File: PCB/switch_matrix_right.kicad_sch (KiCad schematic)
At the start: 78 parts, among them SW41 SW_Push, SW42 SW_Push, SW43 SW_Push, SW44 SW_Push, SW45 SW_Push, SW46 SW_Push, SW47 SW_Push, SW48 SW_Push, SW49 SW_Push, SW50 SW_Push, SW51 SW_Push, SW52 SW_Push, SW53 SW_Push, SW54 SW_Push, SW55 SW_Push, SW56 SW_Push, SW57 SW_Push, SW58 SW_Push, SW59 SW_Push, SW60 SW_Push, SW61 SW_Push, SW62 SW_Push, SW63 SW_Push, SW64 SW_Push, SW65 SW_Push, SW66 SW_Push, SW67 SW_Push, SW68 SW_Push, SW69 SW_Push, SW70 SW_Push, SW71 SW_Push, SW72 SW_Push, SW73 SW_Push, SW74 SW_Push, SW75 SW_Push, SW76 SW_Push, SW77 SW_Push, SW78 SW_Push, SW79 SW_Push

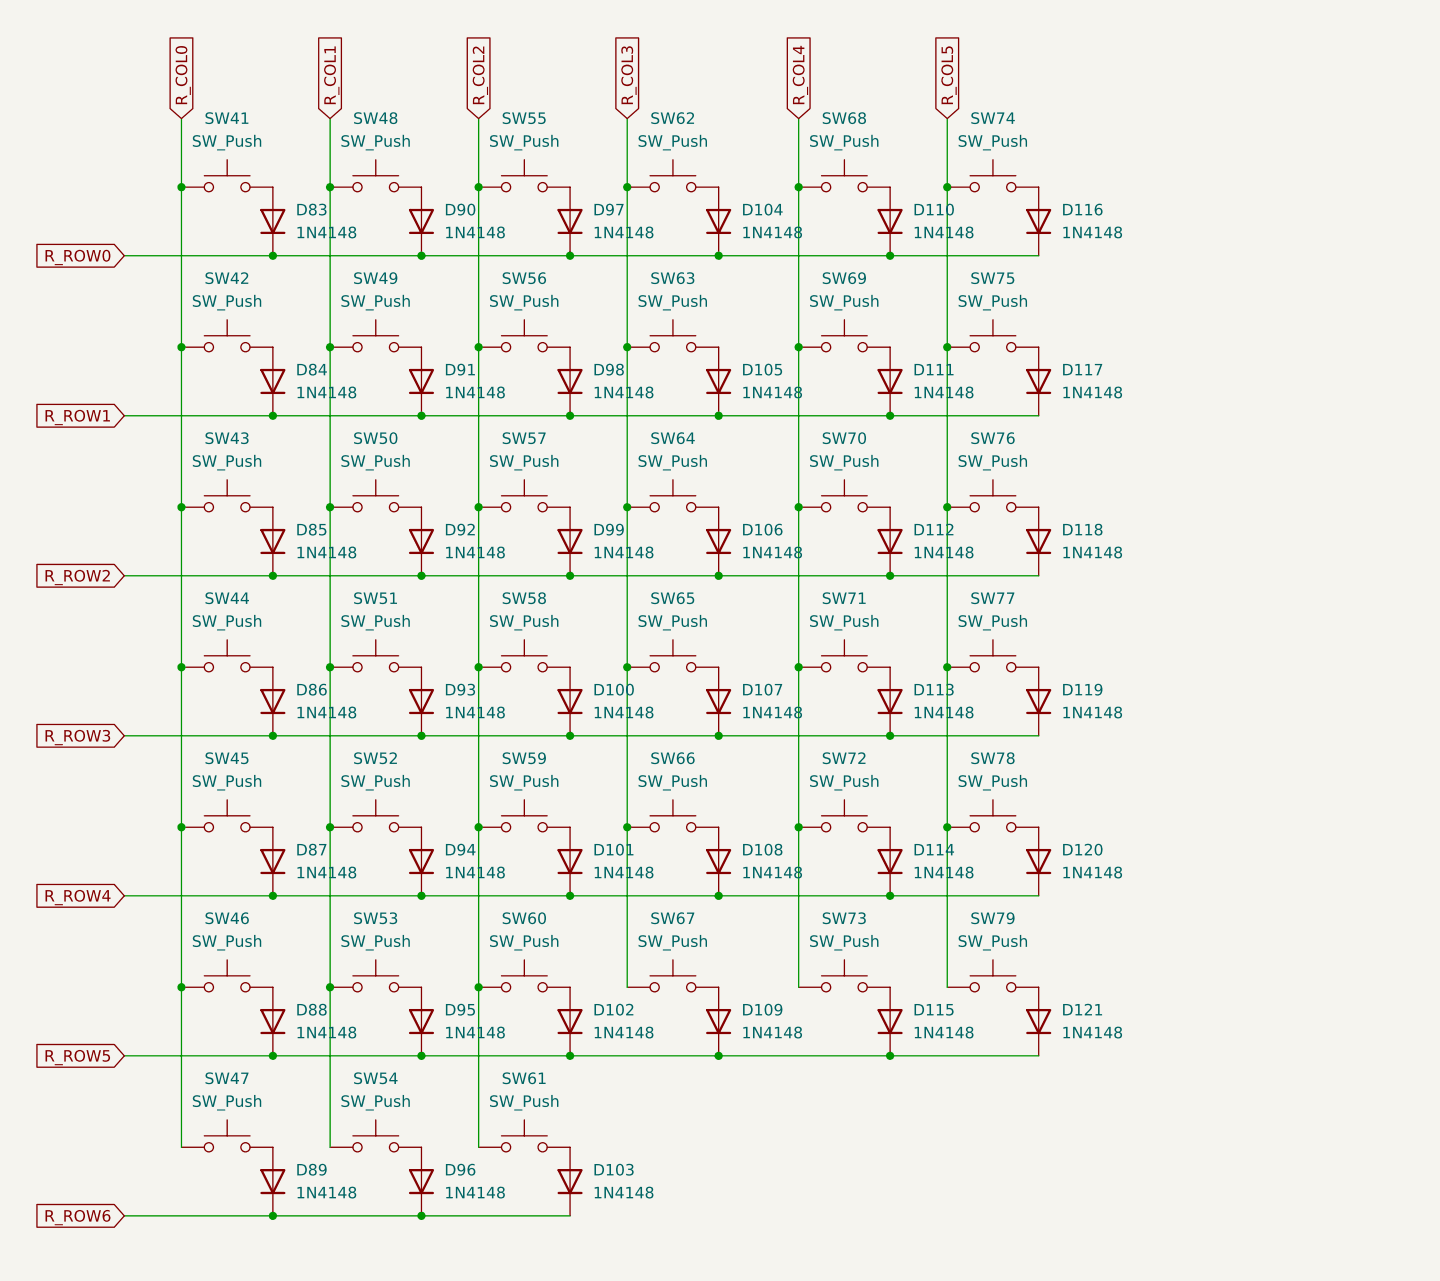
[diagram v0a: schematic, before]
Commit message: updated schematic
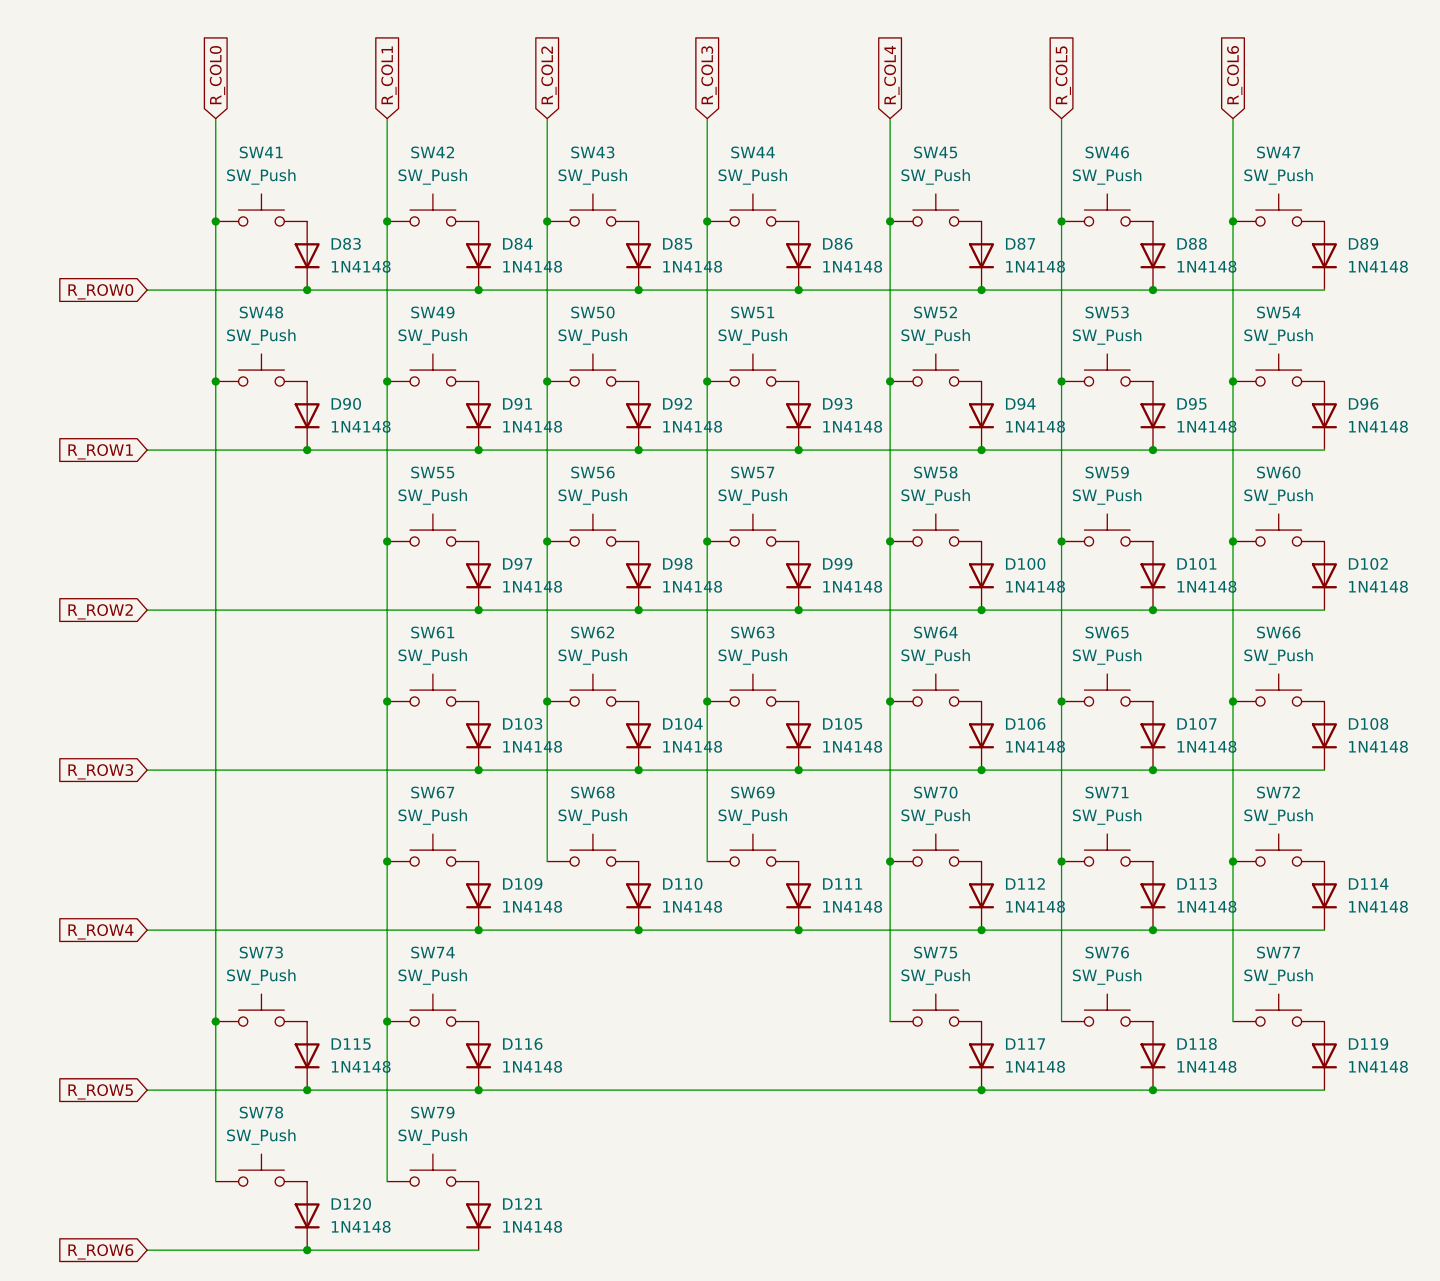
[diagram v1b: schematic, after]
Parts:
- SW41, SW42, SW43, SW44, SW45, SW46, SW47, SW48, SW49, SW50, SW51, SW52, SW53, SW54, SW55, SW56, SW57, SW58, SW59, SW62, SW63, SW64, SW65, SW66, SW67, SW68, SW69, SW70, SW71, SW72, SW73, SW74, SW75: footprint Gateron_KS33_Hotswap:Gateron-KS33-Hotswap-1U -> (none)
- SW60, SW61: footprint Gateron_KS33_Hotswap:Gateron-KS33-Hotswap-2U -> (none)
- SW76, SW77, SW78, SW79: footprint Gateron_KS33_Hotswap:Gateron-KS33-Hotswap-1.25U -> (none)
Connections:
- net R_COL0: now also SW48.1, SW73.1, SW78.1; no longer SW42.1, SW43.1, SW44.1, SW45.1, SW46.1, SW47.1
- net R_COL1: now also SW42.1, SW55.1, SW61.1, SW67.1, SW74.1, SW79.1; no longer SW48.1, SW50.1, SW51.1, SW52.1, SW53.1, SW54.1
- net R_COL2: now also SW43.1, SW50.1, SW62.1, SW68.1; no longer SW55.1, SW57.1, SW58.1, SW59.1, SW60.1, SW61.1
- net R_COL3: now also SW44.1, SW51.1, SW57.1, SW69.1; no longer SW62.1, SW64.1, SW65.1, SW66.1, SW67.1
- net R_COL4: now also SW45.1, SW52.1, SW58.1, SW64.1, SW75.1; no longer SW68.1, SW69.1, SW71.1, SW72.1, SW73.1
- net R_COL5: now also SW46.1, SW53.1, SW59.1, SW65.1, SW71.1; no longer SW74.1, SW75.1, SW77.1, SW78.1, SW79.1
- net R_ROW0: now also D84.1 (K), D85.1 (K), D86.1 (K), D87.1 (K), D88.1 (K), D89.1 (K); no longer D104.1 (K), D110.1 (K), D116.1 (K), D90.1 (K), D97.1 (K)
- net R_ROW1: now also D90.1 (K), D92.1 (K), D93.1 (K), D94.1 (K), D95.1 (K), D96.1 (K); no longer D105.1 (K), D111.1 (K), D117.1 (K), D84.1 (K), D98.1 (K)
- net R_ROW2: now also D100.1 (K), D101.1 (K), D102.1 (K), D97.1 (K), D98.1 (K); no longer D106.1 (K), D112.1 (K), D118.1 (K), D85.1 (K), D92.1 (K)
- net R_ROW3: now also D103.1 (K), D104.1 (K), D105.1 (K), D106.1 (K), D108.1 (K); no longer D100.1 (K), D113.1 (K), D119.1 (K), D86.1 (K), D93.1 (K)
- net R_ROW4: now also D109.1 (K), D110.1 (K), D111.1 (K), D112.1 (K), D113.1 (K); no longer D101.1 (K), D108.1 (K), D120.1 (K), D87.1 (K), D94.1 (K)
- net R_ROW5: now also D116.1 (K), D117.1 (K), D118.1 (K), D119.1 (K); no longer D102.1 (K), D109.1 (K), D121.1 (K), D88.1 (K), D95.1 (K)
- net R_ROW6: now also D120.1 (K), D121.1 (K); no longer D103.1 (K), D89.1 (K), D96.1 (K)
- new net R_COL6: SW47.1, SW54.1, SW60.1, SW66.1, SW72.1, SW77.1

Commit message: routed the switches and diodes
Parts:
- SW41, SW42, SW43, SW44, SW45, SW46, SW47, SW48, SW49, SW50, SW51, SW52, SW53, SW54, SW55, SW56, SW57, SW58, SW59, SW61, SW62, SW63, SW64, SW65, SW67, SW68, SW69, SW70, SW71, SW74, SW75, SW76, SW79: footprint (none) -> Gateron_KS33_Hotswap:Gateron-KS33-Hotswap-1U
- SW60, SW66, SW72, SW77: footprint (none) -> Gateron_KS33_Hotswap:Gateron-KS33-Hotswap-1.25U
- SW73, SW78: footprint (none) -> Gateron_KS33_Hotswap:Gateron-KS33-Hotswap-2U
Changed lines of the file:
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@@
 			)
 		)
-		(property "Footprint" ""
+		(property "Footprint" "Gateron_KS33_Hotswap:Gateron-KS33-Hotswap-1U"
 			(at 96.52 30.48 0)
 			(effects
@@
 			)
 		)
-		(property "Footprint" ""
+		(property "Footprint" "Gateron_KS33_Hotswap:Gateron-KS33-Hotswap-1U"
 			(at 116.84 30.48 0)
 			(effects
@@
 			)
 		)
-		(property "Footprint" ""
+		(property "Footprint" "Gateron_KS33_Hotswap:Gateron-KS33-Hotswap-1U"
 			(at 135.89 66.04 0)
 			(effects
@@
 			)
 		)
-		(property "Footprint" ""
+		(property "Footprint" "Gateron_KS33_Hotswap:Gateron-KS33-Hotswap-1U"
 			(at 96.52 66.04 0)
 			(effects
@@
 			)
 		)
-		(property "Footprint" ""
+		(property "Footprint" "Gateron_KS33_Hotswap:Gateron-KS33-Hotswap-1U"
 			(at 116.84 48.26 0)
 			(effects
@@
 			)
 		)
-		(property "Footprint" ""
+		(property "Footprint" "Gateron_KS33_Hotswap:Gateron-KS33-Hotswap-1U"
 			(at 96.52 83.82 0)
 			(effects
@@
 			)
 		)
-		(property "Footprint" ""
+		(property "Footprint" "Gateron_KS33_Hotswap:Gateron-KS33-Hotswap-1U"
 			(at 78.74 83.82 0)
 			(effects
@@
 			)
 		)
-		(property "Footprint" ""
+		(property "Footprint" "Gateron_KS33_Hotswap:Gateron-KS33-Hotswap-2U"
 			(at 41.91 137.16 0)
 			(effects
@@
 			)
 		)
-		(property "Footprint" ""
+		(property "Footprint" "Gateron_KS33_Hotswap:Gateron-KS33-Hotswap-1U"
 			(at 135.89 83.82 0)
 			(effects
@@
 			)
 		)
-		(property "Footprint" ""
+		(property "Footprint" "Gateron_KS33_Hotswap:Gateron-KS33-Hotswap-1U"
 			(at 116.84 66.04 0)
 			(effects
@@
 			)
 		)
-		(property "Footprint" ""
+		(property "Footprint" "Gateron_KS33_Hotswap:Gateron-KS33-Hotswap-1U"
 			(at 135.89 30.48 0)
 			(effects
@@
 			)
 		)
-		(property "Footprint" ""
+		(property "Footprint" "Gateron_KS33_Hotswap:Gateron-KS33-Hotswap-1.25U"
 			(at 154.94 119.38 0)
 			(effects
@@
 			)
 		)
-		(property "Footprint" ""
+		(property "Footprint" "Gateron_KS33_Hotswap:Gateron-KS33-Hotswap-1U"
 			(at 60.96 66.04 0)
 			(effects
@@
 			)
 		)
-		(property "Footprint" ""
+		(property "Footprint" "Gateron_KS33_Hotswap:Gateron-KS33-Hotswap-1U"
 			(at 96.52 48.26 0)
 			(effects
@@
 			)
 		)
-		(property "Footprint" ""
+		(property "Footprint" "Gateron_KS33_Hotswap:Gateron-KS33-Hotswap-1U"
 			(at 60.96 137.16 0)
 			(effects
@@
 			)
 		)
-		(property "Footprint" ""
+		(property "Footprint" "Gateron_KS33_Hotswap:Gateron-KS33-Hotswap-1U"
 			(at 116.84 119.38 0)
 			(effects
@@
 			)
 		)
-		(property "Footprint" ""
+		(property "Footprint" "Gateron_KS33_Hotswap:Gateron-KS33-Hotswap-1U"
 			(at 116.84 101.6 0)
 			(effects
@@
 			)
 		)
-		(property "Footprint" ""
+		(property "Footprint" "Gateron_KS33_Hotswap:Gateron-KS33-Hotswap-1U"
 			(at 60.96 119.38 0)
 			(effects
@@
 			)
 		)
-		(property "Footprint" ""
+		(property "Footprint" "Gateron_KS33_Hotswap:Gateron-KS33-Hotswap-1U"
 			(at 60.96 83.82 0)
 			(effects
@@
 			)
 		)
-		(property "Footprint" ""
+		(property "Footprint" "Gateron_KS33_Hotswap:Gateron-KS33-Hotswap-1U"
 			(at 78.74 30.48 0)
 			(effects
@@
 			)
 		)
-		(property "Footprint" ""
+		(property "Footprint" "Gateron_KS33_Hotswap:Gateron-KS33-Hotswap-1U"
 			(at 135.89 101.6 0)
 			(effects
@@
 			)
 		)
-		(property "Footprint" ""
+		(property "Footprint" "Gateron_KS33_Hotswap:Gateron-KS33-Hotswap-1.25U"
 			(at 154.94 101.6 0)
 			(effects
@@
 			)
 		)
-		(property "Footprint" ""
+		(property "Footprint" "Gateron_KS33_Hotswap:Gateron-KS33-Hotswap-1U"
 			(at 116.84 83.82 0)
 			(effects
@@
 			)
 		)
-		(property "Footprint" ""
+		(property "Footprint" "Gateron_KS33_Hotswap:Gateron-KS33-Hotswap-2U"
 			(at 41.91 119.38 0)
 			(effects
@@
 			)
 		)
-		(property "Footprint" ""
+		(property "Footprint" "Gateron_KS33_Hotswap:Gateron-KS33-Hotswap-1.25U"
 			(at 154.94 66.04 0)
 			(effects
@@
 			)
 		)
-		(property "Footprint" ""
+		(property "Footprint" "Gateron_KS33_Hotswap:Gateron-KS33-Hotswap-1U"
 			(at 78.74 101.6 0)
 			(effects
@@
 			)
 		)
-		(property "Footprint" ""
+		(property "Footprint" "Gateron_KS33_Hotswap:Gateron-KS33-Hotswap-1U"
 			(at 135.89 48.26 0)
 			(effects
@@
 			)
 		)
-		(property "Footprint" ""
+		(property "Footprint" "Gateron_KS33_Hotswap:Gateron-KS33-Hotswap-1.25U"
 			(at 154.94 83.82 0)
 			(effects
@@
 			)
 		)
-		(property "Footprint" ""
+		(property "Footprint" "Gateron_KS33_Hotswap:Gateron-KS33-Hotswap-1U"
 			(at 78.74 66.04 0)
 			(effects
@@
 			)
 		)
-		(property "Footprint" ""
+		(property "Footprint" "Gateron_KS33_Hotswap:Gateron-KS33-Hotswap-1U"
 			(at 96.52 101.6 0)
 			(effects
@@
 			)
 		)
-		(property "Footprint" ""
+		(property "Footprint" "Gateron_KS33_Hotswap:Gateron-KS33-Hotswap-1U"
 			(at 154.94 48.26 0)
 			(effects
@@
 			)
 		)
-		(property "Footprint" ""
+		(property "Footprint" "Gateron_KS33_Hotswap:Gateron-KS33-Hotswap-1U"
 			(at 154.94 30.48 0)
 			(effects
@@
 			)
 		)
-		(property "Footprint" ""
+		(property "Footprint" "Gateron_KS33_Hotswap:Gateron-KS33-Hotswap-1U"
 			(at 78.74 48.26 0)
 			(effects
@@
 			)
 		)
-		(property "Footprint" ""
+		(property "Footprint" "Gateron_KS33_Hotswap:Gateron-KS33-Hotswap-1U"
 			(at 60.96 48.26 0)
 			(effects
@@
 			)
 		)
-		(property "Footprint" ""
+		(property "Footprint" "Gateron_KS33_Hotswap:Gateron-KS33-Hotswap-1U"
 			(at 41.91 48.26 0)
 			(effects
@@
 			)
 		)
-		(property "Footprint" ""
+		(property "Footprint" "Gateron_KS33_Hotswap:Gateron-KS33-Hotswap-1U"
 			(at 135.89 119.38 0)
 			(effects
@@
 			)
 		)
-		(property "Footprint" ""
+		(property "Footprint" "Gateron_KS33_Hotswap:Gateron-KS33-Hotswap-1U"
 			(at 60.96 30.48 0)
 			(effects
@@
 			)
 		)
-		(property "Footprint" ""
+		(property "Footprint" "Gateron_KS33_Hotswap:Gateron-KS33-Hotswap-1U"
 			(at 41.91 30.48 0)
 			(effects
@@
 			)
 		)
-		(property "Footprint" ""
+		(property "Footprint" "Gateron_KS33_Hotswap:Gateron-KS33-Hotswap-1U"
 			(at 60.96 101.6 0)
 			(effects
